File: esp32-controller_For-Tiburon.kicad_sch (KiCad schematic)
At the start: 8 parts, among them J1 PWR_IN, J2 UART1, J3 UART2, J4 I2C_OLED, J5 I2C_PressureSensor, J6 SD_Card_Receptacle, J7 SP1_2_connector, U1 ESP32-S3-WROOM-1

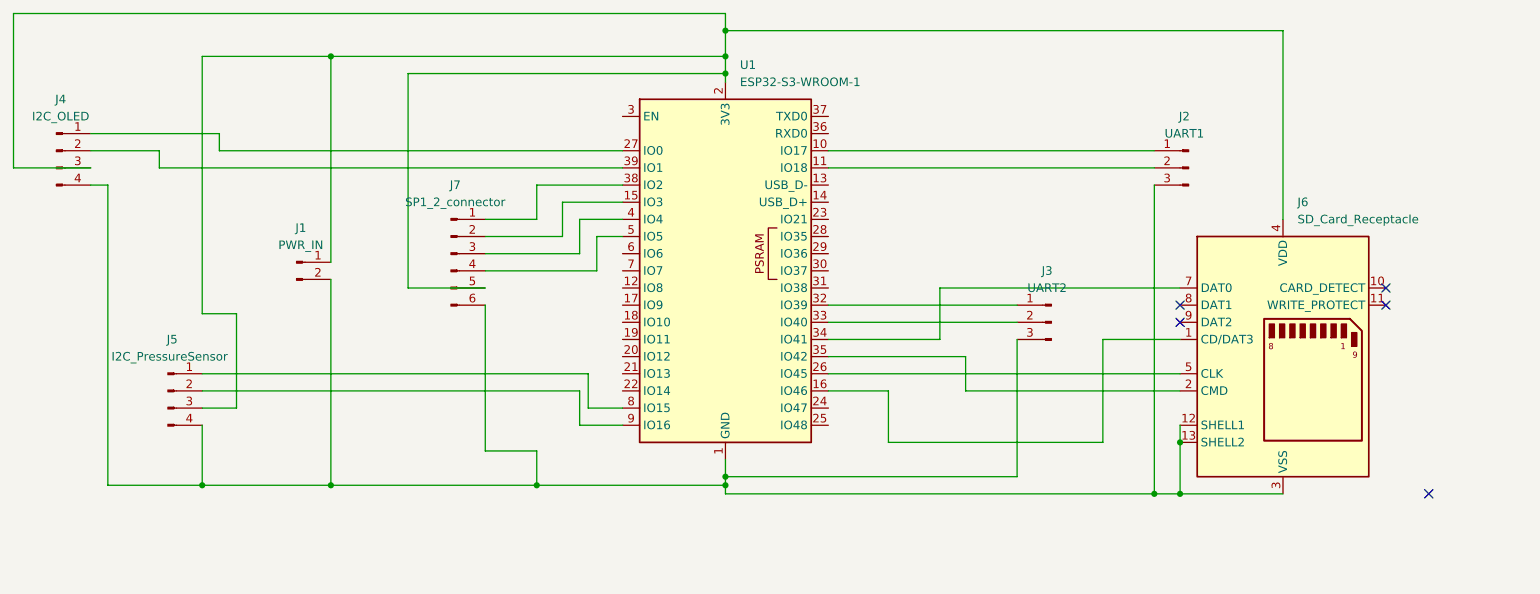
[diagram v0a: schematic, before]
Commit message: Circuit cleanup
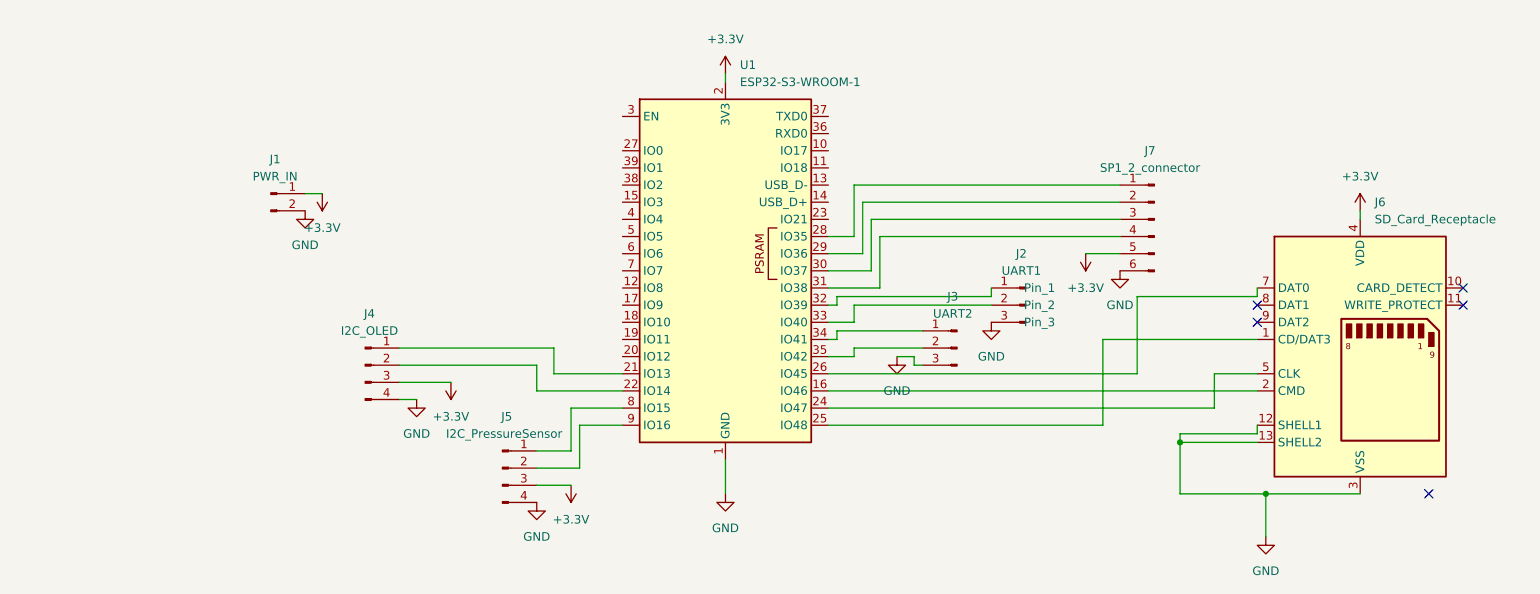
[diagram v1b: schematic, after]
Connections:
- net +3.3V: now reaches J1.1 (Pin_1), J4.3 (Pin_3), J5.3 (Pin_3), J6.4 (VDD), J7.5 (Pin_5), U1.2 (3V3)
- net GND: now reaches J1.2 (Pin_2), J2.3 (Pin_3), J3.3 (Pin_3), J4.4 (Pin_4), J5.4 (Pin_4), J6.12 (SHELL1), J6.13 (SHELL2), J6.3 (VSS), J6.6 (VSS), J7.6 (Pin_6), U1.1 (GND), U1.40 (GND), U1.41 (GND)
- net at J3.1 (Pin_1): now also U1.34 (IO41); no longer U1.32 (IO39)
- net at J3.2 (Pin_2): now also U1.35 (IO42); no longer U1.33 (IO40)
- net at J2.1 (Pin_1): now also U1.32 (IO39); no longer U1.10 (IO17)
- net at J2.2 (Pin_2): now also U1.33 (IO40); no longer U1.11 (IO18)
- net at J7.1 (Pin_1): now also U1.28 (IO35); no longer U1.38 (IO2)
- net at J7.2 (Pin_2): now also U1.29 (IO36); no longer U1.15 (IO3)
- net at J7.3 (Pin_3): now also U1.30 (IO37); no longer U1.4 (IO4)
- net at J7.4 (Pin_4): now also U1.31 (IO38); no longer U1.5 (IO5)
- net at J6.1 (CD/DAT3): now also U1.25 (IO48); no longer U1.16 (IO46)
- net at J6.2 (CMD): now also U1.16 (IO46); no longer U1.35 (IO42)
- net at J6.5 (CLK): now also U1.24 (IO47); no longer U1.26 (IO45)
- net at J6.7 (DAT0): now also U1.26 (IO45); no longer U1.34 (IO41)
- net at U1.21 (IO13): now also J4.1 (Pin_1)
- net at U1.22 (IO14): now also J4.2 (Pin_2)
- net at U1.27 (IO0): no longer J4.1 (Pin_1)
- net at U1.39 (IO1): no longer J4.2 (Pin_2)
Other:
- moved on the sheet: J1, J3, J4, J5, J6, J7
